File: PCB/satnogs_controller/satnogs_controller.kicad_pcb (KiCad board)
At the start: 2 copper layers, 100 x 80 mm, 71 parts, among them P1 DEV-PINS, P2 End-Stops, P3 RJ45, P4 I2C, P7 Motor1, P8 Motor2, U1 ARDUINO_PRO_MINI, U2 MAX485, U3 POLOLU_A4988, U4 POLOLU_A4988, U5 TPS54360DDA, U6 POLOLU_DUAL_MC33926, U7 PCA9540B

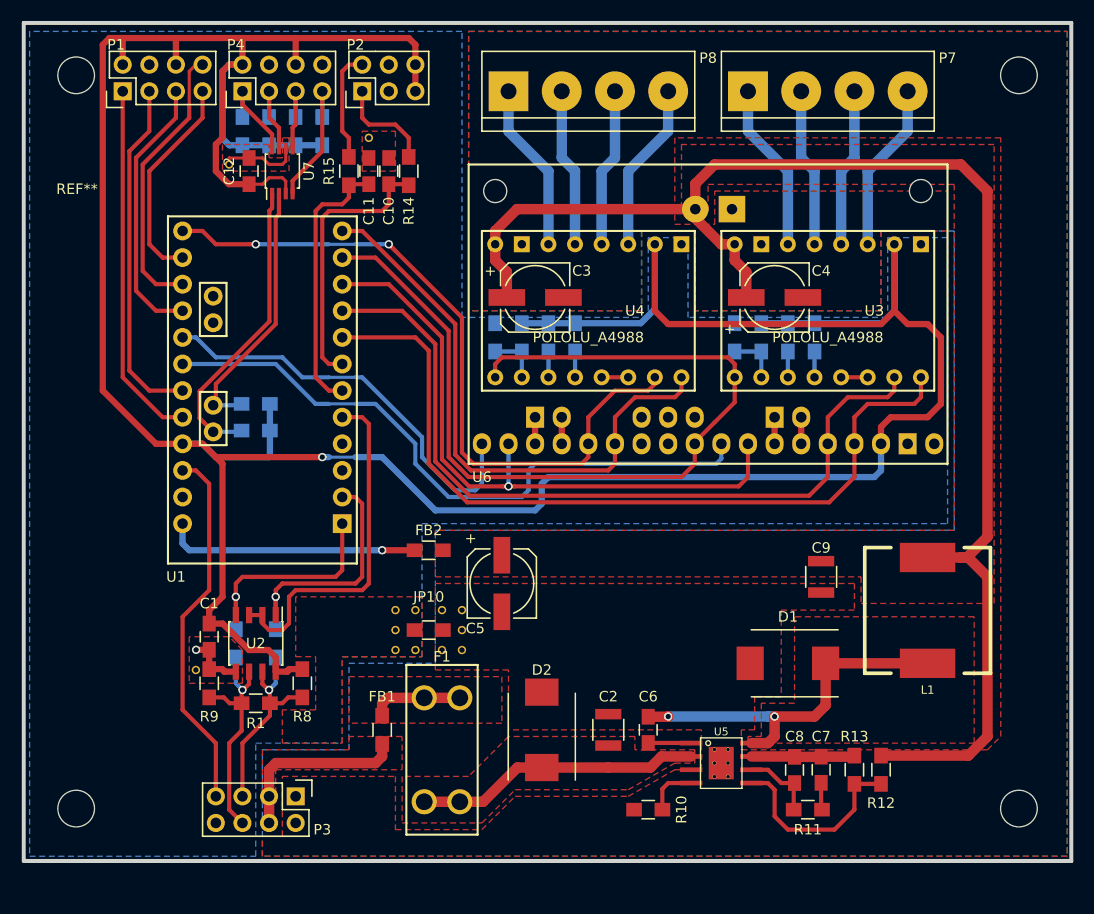
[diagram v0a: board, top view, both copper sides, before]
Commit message: wip
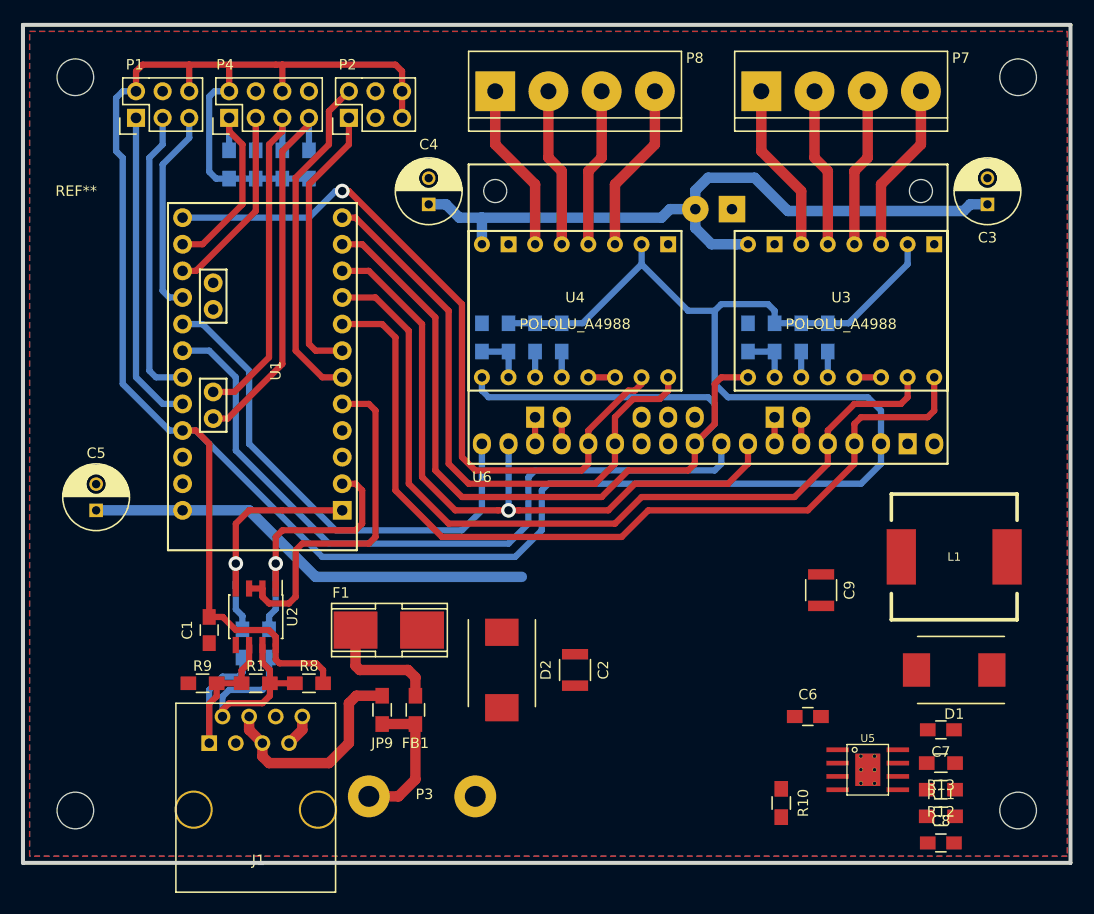
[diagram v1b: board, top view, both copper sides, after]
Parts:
- removed C10, C11, C12: 0.1u, Capacitors_SMD:C_0805_HandSoldering
- removed FB2: FILTER, Resistors_SMD:R_0805_HandSoldering
- removed JP10: Jumper_NO_Small, Resistors_SMD:R_0805_HandSoldering
- removed R14, R15: 200, Resistors_SMD:R_0805_HandSoldering
- removed R16, R17: 4.7k, Resistors_SMD:R_0805_HandSoldering
- removed the REF** at (128.9, 101.6)
- removed the REF** at (127.0, 101.6)
- removed the REF** at (127.0, 97.8)
- removed the REF** at (128.9, 97.8)
- removed the REF** at (131.4, 97.8)
- removed the REF** at (111.1, 55.2)
- removed the REF** at (124.5, 52.7)
- removed the REF** at (127.0, 99.7)
- removed the REF** at (108.0, 103.5)
- removed the REF** at (131.4, 101.6)
- removed the REF** at (133.3, 101.6)
- removed the REF** at (133.3, 99.7)
- removed the REF** at (133.3, 97.8)
- removed U7: PCA9540B, Housings_SSOP:TSSOP-8_3x3mm_Pitch0.65mm
- added J1: RJ45, Connect:RJ45_8, F.Cu at (113.7, 116.8)
- added JP9: Jumper_NO_Small, Resistors_SMD:R_0805_HandSoldering, F.Cu at (125.7, 107.3)
- C3, C4, C5: footprint Capacitors_SMD:c_elec_6.3x5.3 -> Capacitors_ThroughHole:C_Radial_D6.3_L11.2_P2.5
- F1: footprint satnogs:mini-fuse-holder-3568 -> SMD_Packages:Fuse_SMD
- P1: value DEV-PINS -> Dev-Pins; footprint Pin_Headers:Pin_Header_Straight_2x04 -> Pin_Headers:Pin_Header_Straight_2x03
- P3: value RJ45 -> Power-In; footprint Pin_Headers:Pin_Header_Straight_2x04 -> Wire_Connections_Bridges:WireConnection_2.00mmDrill
- moved C3 44.1 mm to (183.5, 59.1), turned to 90 degrees
- moved C5 39.4 mm to (98.4, 88.3), turned to 90 degrees
- moved C4 34.2 mm to (130.2, 59.1), turned to 90 degrees
- moved P3 17.1 mm to (134.6, 115.6), turned to 180 degrees
- moved D1 15.9 mm to (180.3, 103.5)
- moved C8 15.6 mm to (179.1, 120.0), turned to 0 degrees
- moved C6 15.3 mm to (166.4, 108.0), turned to 0 degrees
- moved U5 14.0 mm to (172.1, 113.0)
- moved R10 12.7 mm to (163.8, 116.2), turned to 270 degrees
- moved R11 12.7 mm to (179.1, 117.5)
- moved F1 12.5 mm to (126.4, 99.7), turned to 90 degrees
- moved C7 12.0 mm to (179.1, 109.2), turned to 180 degrees
- moved R13 8.28 mm to (179.1, 112.4), turned to 180 degrees
- moved D2 6.87 mm to (137.2, 103.5), turned to 270 degrees
- moved C2 6.54 mm to (144.1, 103.5), turned to 270 degrees
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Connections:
- net /BOOT renamed Net-(C6-Pad1)
- net /COMP renamed Net-(C8-Pad1)
- net /RT/CLK renamed Net-(R10-Pad1)
- net /SW renamed Net-(C6-Pad2)
- net /SW_VIN renamed Net-(C2-Pad1)
- C1 pad 1: GNDD -> GND
- P1 pad 4: GNDD -> GND
- P2 pad 1: /SW1 -> /SW2
- P2 pad 2: /SW2 -> /SW1
- P2 pad 3: GNDD -> GND
- P2 pad 4: GNDD -> GND
- P3 pad 2: GND -> /VIN
- P4 pad 1: /SCL1 -> /SDA2
- P4 pad 3: /SDA1 -> /SCL2
- P4 pad 4: GNDD -> GND
- P4 pad 5: /SCL0 -> /SDA1
- P4 pad 7: /SDA0 -> /SCL1
- P4 pad 8: GNDD -> GND
- R2 pad 2: /SDA0 -> /SDA1
- R3 pad 2: /SCL0 -> /SCL1
- R4 pad 2: GNDD -> GND
- R5 pad 2: /SDA1 -> /SDA2
- R6 pad 2: /SCL1 -> /SCL2
- R7 pad 2: GNDD -> GND
- R9 pad 2: GNDD -> GND
- U1 pad 14: /PB3 -> /SDA2
- U1 pad 15: /PB4 -> /SCL2
- U1 pad 23: /SDA -> /SDA1
- U1 pad 24: /SCL -> /SCL1
- U1 pad 26: /RST -> Net-(U1-Pad26)
- U1 pad 27: GNDD -> GND
- U1 pad 28: Net-(FB2-Pad1) -> +12V
- U1 pad 4: GNDD -> GND
- U1 pad 6: /SW2_F -> /SW1
- U1 pad 7: /SW1_F -> /SW2
- U2 pad 5: GNDD -> GND
- U3 pad 1: GNDD -> GND
- U4 pad 1: GNDD -> GND
- U6 pad 2: GNDD -> GND
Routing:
- net +5V: track 339.5 -> 288.2 mm, vias 1 -> 0
- net Net-(C6-Pad2): track 35.5 -> 0.00 mm, vias 2 -> 0
- net /RST: track 35.3 -> 0.00 mm
- net /SCL: track 28.7 -> 0.00 mm
- net +12V: track 139.4 -> 111.3 mm
- net /SCL1: track 9.10 -> 36.4 mm
- net Net-(C2-Pad1): track 27.3 -> 0.00 mm
- net /PB4: track 26.8 -> 0.00 mm
- net /SW1_F: track 26.3 -> 0.00 mm
- net /SW2_F: track 25.8 -> 0.00 mm
- net /SDA: track 25.4 -> 0.00 mm
- net /SDA1: track 8.32 -> 33.2 mm
- net Net-(FB2-Pad1): track 24.3 -> 0.00 mm, vias 1 -> 0
- net /SW1: track 9.60 -> 32.4 mm
- net /SCL2: track 0.00 -> 21.3 mm
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- removed copper zone on F.Cu, net +12V
- removed copper zone on F.Cu, net /VIN
- removed copper zone on B.Cu, net GNDD
- removed copper zone on F.Cu, net GNDD
- removed copper zone on F.Cu, net Net-(C2-Pad1)
- removed copper zone on F.Cu, net Net-(C6-Pad2)
- removed copper zone on F.Cu, net Net-(F1-Pad1)
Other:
- net class Default: via_dia 0.8 -> 1.4; via_drill 0.5 -> 0.8
- net class neck removed
- net class power added: clearance 0.2, trace_width 1, via_dia 1.4, via_drill 0.8
- net class power1 removed
- net class power2 removed
- net class power_low added: clearance 0.2, trace_width 0.6, via_dia 1.4, via_drill 0.8
- net class signal: trace_width 0.4 -> 0.6; via_dia 0.8 -> 1.4; via_drill 0.5 -> 0.8
